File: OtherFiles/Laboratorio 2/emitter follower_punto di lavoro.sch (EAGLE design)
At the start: 4 parts

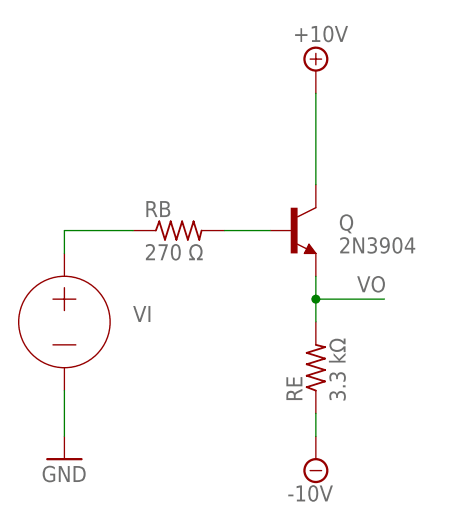
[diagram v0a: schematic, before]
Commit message: continuato analisi laboratorio 2
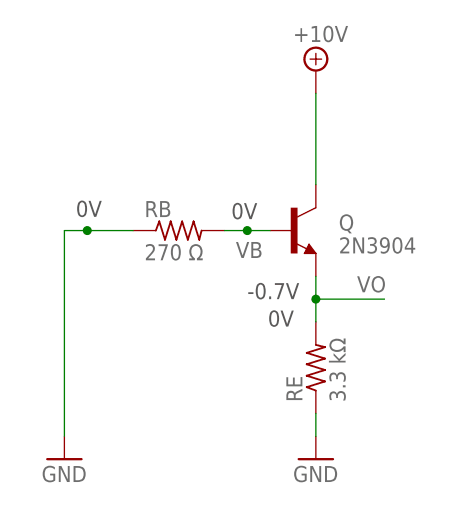
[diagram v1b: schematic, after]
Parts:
- removed VI: 0V, ngspice-simulation:VOLTAGE
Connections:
- removed net -10V: RE.1
- removed net N$3: RB.1, VI.+
- net GND: now also RB.1, RE.1; no longer VI.-
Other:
- note added: "-0.7V"
- note added: "0V"
- note added: "VB"
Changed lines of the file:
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@@
 <part name="Q" library="transistor" library_urn="urn:adsk.eagle:library:402" deviceset="2N3904" device="" package3d_urn="urn:adsk.eagle:package:28523/2"/>
 <part name="RB" library="rcl" library_urn="urn:adsk.eagle:library:334" deviceset="R-US_" device="0204/5" package3d_urn="urn:adsk.eagle:package:23488/1" value="270 Ω"/>
-<part name="VI" library="ngspice-simulation" library_urn="urn:adsk.eagle:library:527439" deviceset="VOLTAGE" device="" value="0V"/>
 <part name="RE" library="rcl" library_urn="urn:adsk.eagle:library:334" deviceset="R-US_" device="0204/5" package3d_urn="urn:adsk.eagle:package:23488/1" value="3.3 kΩ"/>
 <part name="GND1" library="supply1" library_urn="urn:adsk.eagle:library:371" deviceset="GND" device=""/>
 <part name="SUPPLY1" library="supply2" library_urn="urn:adsk.eagle:library:372" deviceset="+10V" device=""/>
-<part name="SUPPLY2" library="supply2" library_urn="urn:adsk.eagle:library:372" deviceset="-10V" device=""/>
+<part name="GND2" library="supply1" library_urn="urn:adsk.eagle:library:371" deviceset="GND" device=""/>
 </parts>
 <sheets>
 <sheet>
 <plain>
+<text x="29.21" y="42.164" size="1.778" layer="92">0V</text>
+<text x="46.482" y="41.91" size="1.778" layer="92">0V</text>
+<text x="48.26" y="33.02" size="1.778" layer="92">-0.7V</text>
+<text x="50.546" y="29.972" size="1.778" layer="92">0V</text>
+<text x="46.99" y="37.592" size="1.778" layer="95">VB</text>
 </plain>
 <instances>
@@
 <attribute name="NAME" x="36.83" y="42.1386" size="1.778" layer="95"/>
 <attribute name="VALUE" x="36.83" y="37.338" size="1.778" layer="96"/>
-</instance>
-<instance part="VI" gate="G$1" x="27.94" y="30.48" smashed="yes">
-<attribute name="NAME" x="35.56" y="30.48" size="1.778" layer="95"/>
 </instance>
 <instance part="RE" gate="G$1" x="55.88" y="25.4" smashed="yes" rot="R90">
@@
 <attribute name="VALUE" x="53.34" y="61.595" size="1.778" layer="96"/>
 </instance>
-<instance part="SUPPLY2" gate="G$1" x="55.88" y="15.24" smashed="yes">
-<attribute name="VALUE" x="52.705" y="10.541" size="1.778" layer="96"/>
+<instance part="GND2" gate="1" x="55.88" y="15.24" smashed="yes">
+<attribute name="VALUE" x="53.34" y="12.7" size="1.778" layer="96"/>
 </instance>
 </instances>
@@
 <pinref part="Q" gate="G1" pin="B"/>
 <pinref part="RB" gate="G$1" pin="2"/>
-<wire x1="50.8" y1="40.64" x2="45.72" y2="40.64" width="0.1524" layer="91"/>
-</segment>
-</net>
-<net name="N$3" class="0">
-<segment>
-<pinref part="VI" gate="G$1" pin="+"/>
-<pinref part="RB" gate="G$1" pin="1"/>
-<wire x1="27.94" y1="38.1" x2="27.94" y2="40.64" width="0.1524" layer="91"/>
-<wire x1="27.94" y1="40.64" x2="35.56" y2="40.64" width="0.1524" layer="91"/>
+<wire x1="50.8" y1="40.64" x2="48.26" y2="40.64" width="0.1524" layer="91"/>
+<junction x="48.26" y="40.64"/>
+<wire x1="48.26" y1="40.64" x2="45.72" y2="40.64" width="0.1524" layer="91"/>
 </segment>
 </net>
 <net name="GND" class="0">
 <segment>
-<pinref part="VI" gate="G$1" pin="-"/>
 <pinref part="GND1" gate="1" pin="GND"/>
-<wire x1="27.94" y1="22.86" x2="27.94" y2="17.78" width="0.1524" layer="91"/>
+<pinref part="RB" gate="G$1" pin="1"/>
+<wire x1="27.94" y1="40.64" x2="30.48" y2="40.64" width="0.1524" layer="91"/>
+<wire x1="30.48" y1="40.64" x2="35.56" y2="40.64" width="0.1524" layer="91"/>
+<wire x1="27.94" y1="40.64" x2="27.94" y2="17.78" width="0.1524" layer="91"/>
+<junction x="30.48" y="40.64"/>
+</segment>
+<segment>
+<pinref part="RE" gate="G$1" pin="1"/>
+<wire x1="55.88" y1="17.78" x2="55.88" y2="20.32" width="0.1524" layer="91"/>
+<pinref part="GND2" gate="1" pin="GND"/>
 </segment>
 </net>
@@
 </segment>
 </net>
-<net name="-10V" class="0">
-<segment>
-<pinref part="RE" gate="G$1" pin="1"/>
-<wire x1="55.88" y1="17.78" x2="55.88" y2="20.32" width="0.1524" layer="91"/>
-<pinref part="SUPPLY2" gate="G$1" pin="-10V"/>
-</segment>
-</net>
